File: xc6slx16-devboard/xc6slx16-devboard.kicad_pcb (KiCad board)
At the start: 4 copper layers, 75 x 65 mm, 141 parts, among them IC1 LM26480, IC2 M25P80-VMN6P, IC3 25MHz, IC4 SOT95P275X110-5N, IC5 SOT95P275X110-5N, J1 10118241-001RLF, J2 Conn_02x15_Odd_Even, J3 Conn_02x05_Odd_Even, J4 Conn_02x15_Odd_Even, J5 USB_C, Q1 2N7002, Q2 2N7002, Q3 Q_BSS84, Q4 2N7002, SW1 SW_Push, U1 XC6SLX16-FTG256, U2 K4X1G163PE, U3 CH340E

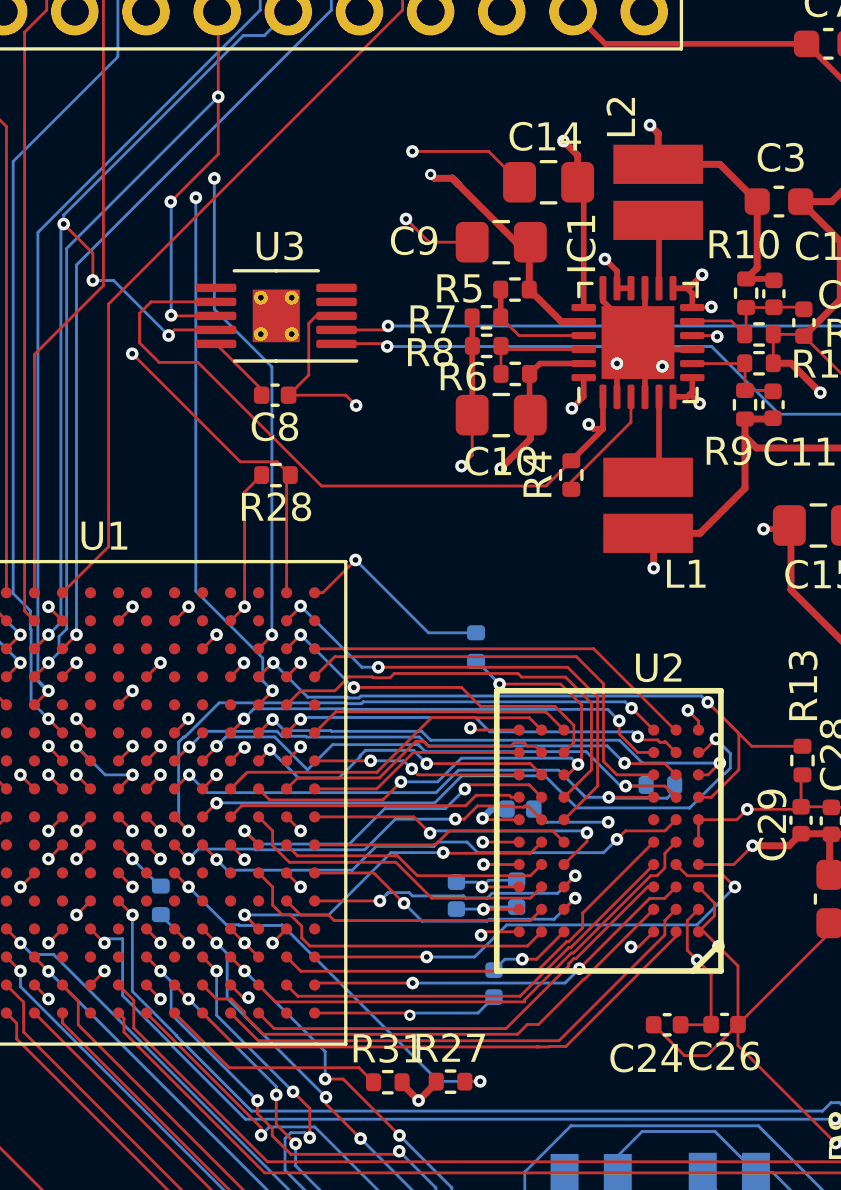
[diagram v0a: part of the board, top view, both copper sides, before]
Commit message: gerber
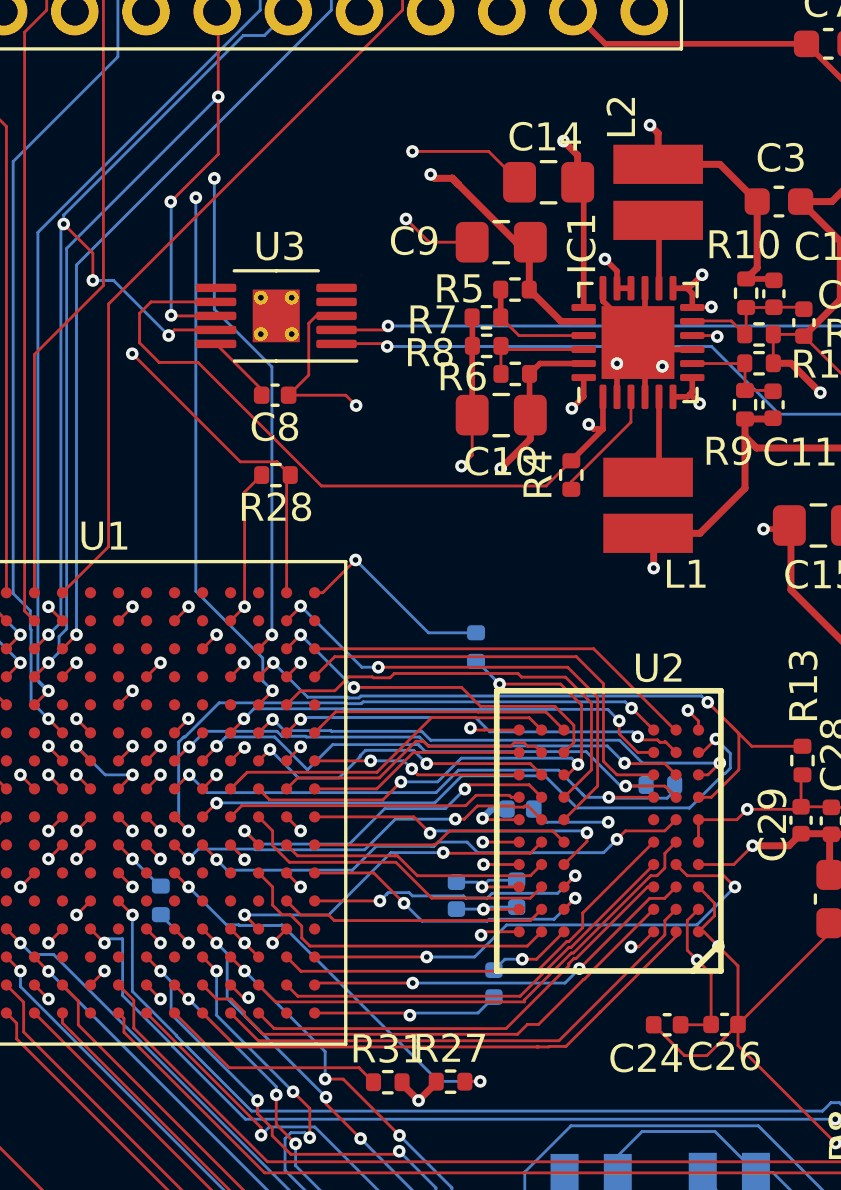
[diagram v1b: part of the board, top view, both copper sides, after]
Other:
- net class 2: via_dia 0.4 -> 0.45
- net class Default: via_dia 0.4 -> 0.45
- rule via_min_size: 0.4 -> 0.45
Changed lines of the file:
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@@
-(kicad_pcb (version 20171130) (host pcbnew "(5.1.7-0-10_14)")
+(kicad_pcb (version 20171130) (host pcbnew "(5.1.8-0-10_14)")
   (general
     (thickness 1.6)
@@
     (zone_45_only no)
     (trace_min 0.1016)
-    (via_size 0.4)
+    (via_size 0.45)
     (via_drill 0.2)
-    (via_min_size 0.4)
+    (via_min_size 0.45)
     (via_min_drill 0.2)
-    (uvia_size 0.4)
+    (uvia_size 0.45)
     (uvia_drill 0.2)
     (uvias_allowed no)
-    (uvia_min_size 0.4)
+    (uvia_min_size 0.45)
     (uvia_min_drill 0.2)
     (edge_width 0.05)
@@
       (drillshape 0)
       (scaleselection 1)
-      (outputdirectory "xc64lx16-devboard/"))
+      (outputdirectory "xc6slx16-devboard/"))
   )
   (net 0 "")
@@
     (clearance 0.1016)
     (trace_width 0.1016)
-    (via_dia 0.4)
+    (via_dia 0.45)
     (via_drill 0.2)
-    (uvia_dia 0.4)
+    (uvia_dia 0.45)
     (uvia_drill 0.2)
     (diff_pair_width 0.1016)
@@
     (clearance 0.2032)
     (trace_width 0.2032)
-    (via_dia 0.4)
+    (via_dia 0.45)
     (via_drill 0.2)
-    (uvia_dia 0.4)
+    (uvia_dia 0.45)
     (uvia_drill 0.2)
   )
@@
   (segment (start 167.955 88.9) (end 166.771446 88.9) (width 0.1016) (layer F.Cu) (net 2))
   (segment (start 147.61 81.48) (end 148.18 80.91) (width 0.1016) (layer B.Cu) (net 2))
-  (via (at 145.18 81.56) (size 0.4) (drill 0.2) (layers F.Cu B.Cu) (net 2))
+  (via (at 145.18 81.56) (size 0.45) (drill 0.2) (layers F.Cu B.Cu) (net 2))
   (segment (start 145.3 81.48) (end 145.26 81.48) (width 0.1016) (layer B.Cu) (net 2))
   (segment (start 145.26 81.48) (end 145.18 81.56) (width 0.1016) (layer B.Cu) (net 2))
@@
   (segment (start 146.06 51.69) (end 145.92 51.55) (width 0.25) (layer F.Cu) (net 28))
   (segment (start 145.92 51.55) (end 145.92 61.34) (width 0.25) (layer L3) (net 28))
-  (via (at 145.92 51.55) (size 0.4) (drill 0.2) (layers F.Cu B.Cu) (net 28))
+  (via (at 145.92 51.55) (size 0.45) (drill 0.2) (layers F.Cu B.Cu) (net 28))
   (segment (start 146.69 51.69) (end 146.06 51.69) (width 0.25) (layer F.Cu) (net 28))
   (segment (start 145.92 45.74) (end 145.92 51.55) (width 0.25) (layer L3) (net 28))

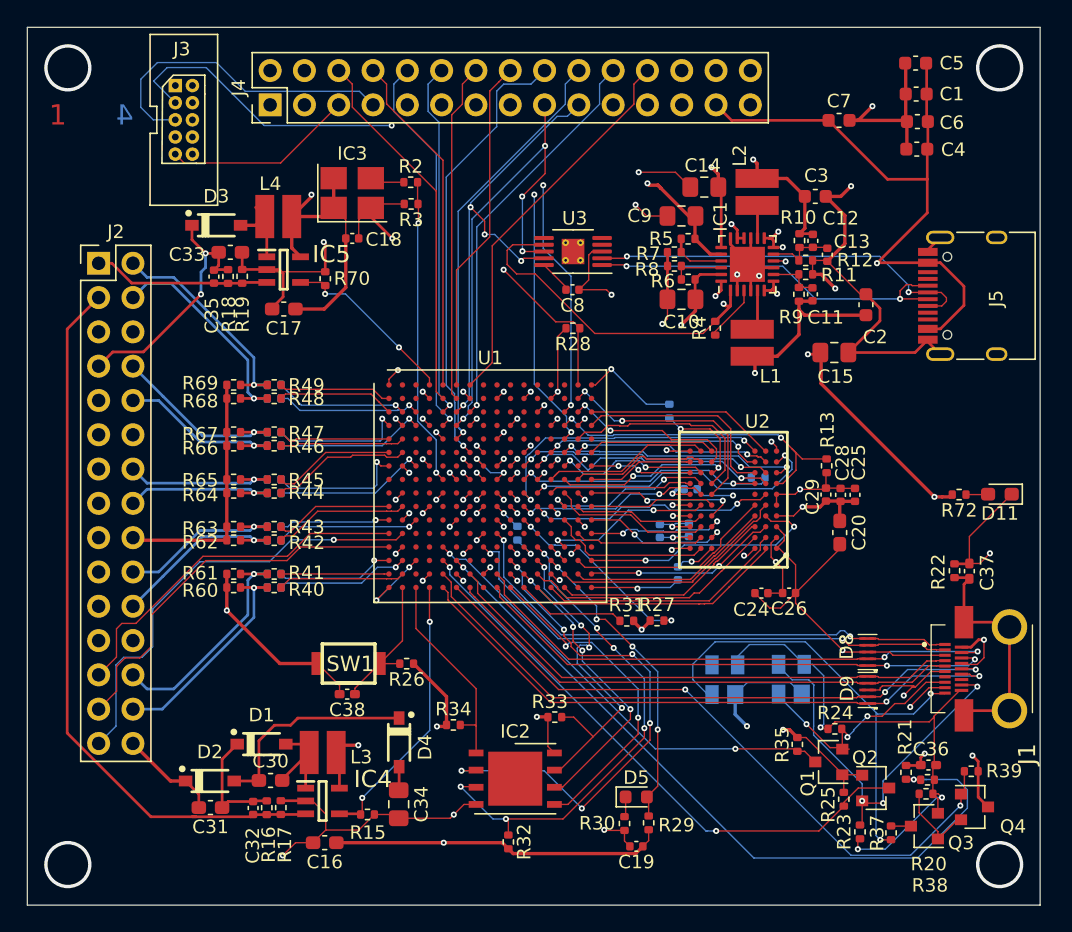
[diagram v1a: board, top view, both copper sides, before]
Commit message: xc6slx16-rev2
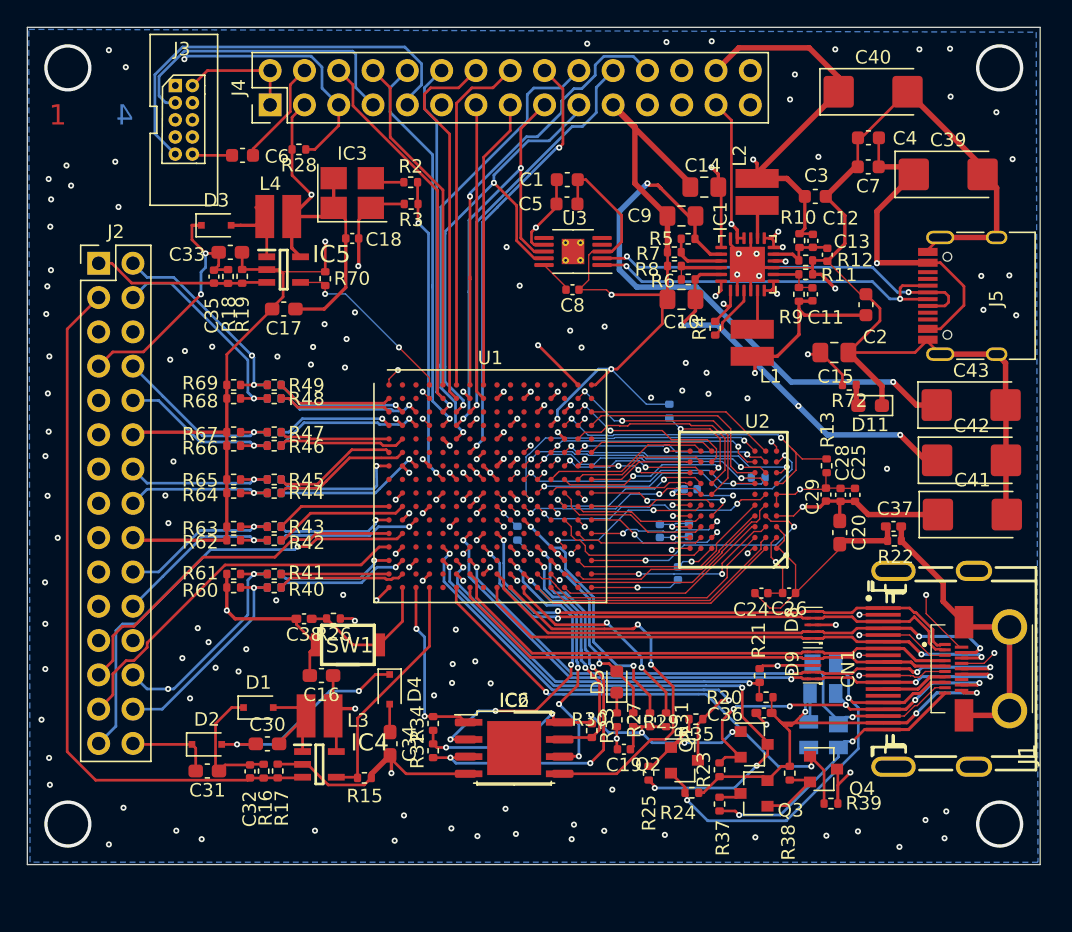
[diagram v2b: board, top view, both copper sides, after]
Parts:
- added C39: CP, Capacitor_Tantalum_SMD:CP_EIA-6032-28_Kemet-C_Pad2.25x2.35mm_HandSolder, F.Cu at (168.2, 50.9)
- added C40: CP, Capacitor_Tantalum_SMD:CP_EIA-6032-28_Kemet-C_Pad2.25x2.35mm_HandSolder, F.Cu at (162.6, 44.8)
- added C41: CP, Capacitor_Tantalum_SMD:CP_EIA-6032-28_Kemet-C_Pad2.25x2.35mm_HandSolder, F.Cu at (170.0, 76.1)
- added C42: CP, Capacitor_Tantalum_SMD:CP_EIA-6032-28_Kemet-C_Pad2.25x2.35mm_HandSolder, F.Cu at (169.9, 72.1)
- added C43: CP, Capacitor_Tantalum_SMD:CP_EIA-6032-28_Kemet-C_Pad2.25x2.35mm_HandSolder, F.Cu at (169.9, 68.0)
- added CN1: Connector_HDMI_19_Male_+_1_Shield, dsi_shield:MOLEX_500254-1927, F.Cu at (163.4, 87.5)
- added IC6: M25P80-VMN6P, Package_SO:SOP-8_5.28x5.23mm_P1.27mm, F.Cu at (136.1, 93.4)
- C34: footprint Capacitor_SMD:C_0805_2012Metric_Pad1.18x1.45mm_HandSolder -> Capacitor_SMD:C_0603_1608Metric_Pad1.08x0.95mm_HandSolder
- C38: value C -> 100n
- D1, D2, D3, D4: value Diode_Schottky -> 1N4148; footprint dsi_shield:SOD3715X145N -> Diode_SMD:D_SOD-323F
- IC4, IC5: value SOT95P275X110-5N -> TPS61040
- moved C6 50.0 mm to (115.9, 49.5)
- moved C5 27.8 mm to (140.0, 53.1), turned to 0 degrees
- moved C1 26.6 mm to (140.0, 51.3), turned to 180 degrees
- moved R28 24.2 mm to (120.1, 49.0)
- moved R25 14.6 mm to (146.0, 95.2)
- moved R20 13.4 mm to (154.7, 89.6)
- moved R21 13.0 mm to (154.2, 88.0)
- moved R37 12.9 mm to (151.3, 97.5)
- moved Q3 12.8 mm to (153.8, 96.7)
- moved C36 12.8 mm to (154.6, 90.8)
- moved C16 12.4 mm to (121.8, 88.0)
- moved D11 11.6 mm to (162.4, 68.0)
- moved R24 11.6 mm to (149.2, 96.7), turned to 180 degrees
- moved Q4 11.5 mm to (159.0, 94.9)
- moved R72 11.5 mm to (160.9, 66.5)
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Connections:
- J4 pad 13: SCL -> DBG_SCL
- J4 pad 15: SDA -> DBG_SDA
- J4 pad 3: +5V -> +3V3
- J4 pad 4: +3V3 -> +5V
- J4 pad 5: FPGA_TDI -> FPGA_TMS
- J4 pad 7: FPGA_TMS -> FPGA_TDO
- J4 pad 9: FPGA_TDO -> FPGA_TDI
- U1 pad A8: Net-(U1-PadA8) -> DBG_SDA
- U1 pad B8: Net-(U1-PadB8) -> DBG_SCL
- U1 pad M7: Net-(U1-PadM7) -> /hdmi-in/TMDS_CLK_N
- U1 pad P7: Net-(U1-PadP7) -> /hdmi-in/TMDS_CLK_P
- U1 pad R5: /hdmi-in/TMDS_CLK_P -> Net-(U1-PadR5)
- U1 pad T5: /hdmi-in/TMDS_CLK_N -> Net-(U1-PadT5)
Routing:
- net GND: track 330.4 -> 726.5 mm, vias 56 -> 155
- net +3V3: track 351.3 -> 296.2 mm, vias 20 -> 22
- net +1V2: track 59.6 -> 93.3 mm
- net /hdmi-in/MH1: track 0.00 -> 31.5 mm
- net /hdmi-in/HPD_NOTIFY: track 57.0 -> 28.7 mm
- net DBG_SCL: track 0.00 -> 22.0 mm
- net DBG_SDA: track 0.00 -> 21.6 mm
- net +2V5: track 94.6 -> 114.9 mm, vias 9 -> 11
- net HDMI_HPD: track 35.7 -> 21.0 mm
- net HDMI_SCL: track 18.3 -> 32.9 mm, vias 3 -> 2
- net /xc6slx16/QSPI_DQ1: track 38.3 -> 23.8 mm, vias 6 -> 4
- net /hdmi-in/HPD_EN: track 49.7 -> 37.2 mm
- net +5V: track 134.5 -> 123.9 mm, vias 7 -> 8
- net FPGA_TDI: track 50.3 -> 59.1 mm
- net Net-(D5-Pad2): track 23.0 -> 14.2 mm, vias 4 -> 2
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- added copper zone on B.Cu, net GND
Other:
- board size 75 x 65 mm -> 75 x 62 mm
